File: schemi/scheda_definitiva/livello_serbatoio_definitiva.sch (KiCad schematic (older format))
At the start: 46 parts, among them J1 USB_B, J2 BTN_LED_GROUP, J3 CONN_LCD, J4 CONN_US, J5 ICSP, J6 Exp_Analog_2, J7 Exp_Analog, SW1 SW_RST, U1 FT232RL, U2 ATmega328P-PU, U3 USBLC6-2SC6, Y1 16MHz

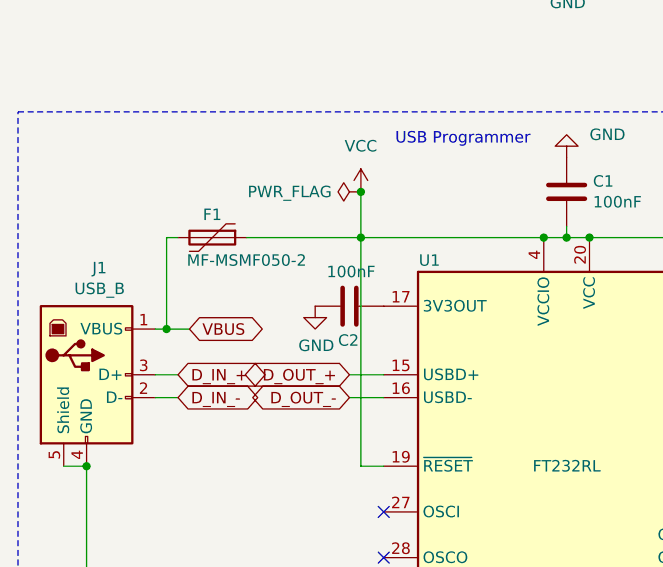
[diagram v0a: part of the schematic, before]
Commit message: aggiunta ferrite a scheda rev. B
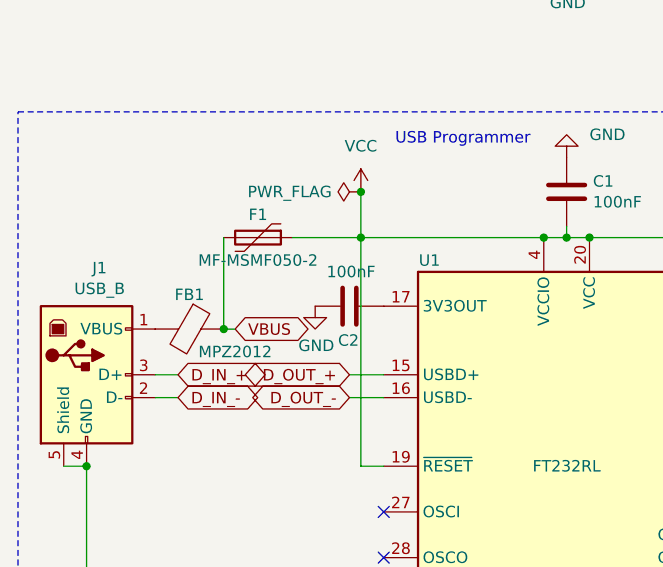
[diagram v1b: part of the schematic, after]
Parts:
- added FB1: MPZ2012, Inductor_SMD:L_0805_2012Metric_Pad1.15x1.40mm_HandSolder, symbol Device:Ferrite_Bead
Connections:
- net VBUS: now also FB1.1; no longer J1.1 (VBUS)
- new net: FB1.2, J1.1 (VBUS)
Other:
- moved on the sheet: F1
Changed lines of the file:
@@
 	0    -1   -1   0
 $EndComp
-Wire Wire Line
-	1250 2750 1300 2750
-Connection ~ 1300 2750
-Wire Wire Line
-	1300 2350 1300 2750
 $Comp
 L Device:R R9
@@
 DTR
 Wire Wire Line
-	1650 2350 2150 2350
-Wire Wire Line
 	2150 2150 2150 2350
 NoConn ~ 2250 3750
@@
 Wire Wire Line
 	2250 3350 2150 3350
-Wire Wire Line
-	1300 2350 1350 2350
 $Comp
 L Device:C C2
@@
 Text GLabel 1350 3050 2    50   BiDi ~ 0
 D_IN_-
-Text GLabel 1400 2750 2    50   BiDi ~ 0
-VBUS
 Text GLabel 2100 2950 0    50   BiDi ~ 0
 D_OUT_+
@@
 Text GLabel 2050 5700 2    50   BiDi ~ 0
 D_OUT_-
-Wire Wire Line
-	1300 2750 1400 2750
 Wire Wire Line
 	1250 2950 1350 2950
@@
 L Device:Polyfuse F1
 U 1 1 5FB200DA
-P 1500 2350
-F 0 "F1" V 1400 2350 50  0000 C CNN
-F 1 "MF-MSMF050-2" V 1600 2500 50  0000 C CNN
-F 2 "simboli_custom:MF-MSMF_1812_4532Metric_Pad1.30x3.40mm_HandSolder" H 1550 2150 50  0001 L CNN
-F 3 "~" H 1500 2350 50  0001 C CNN
-	1    1500 2350
+P 1700 2350
+F 0 "F1" V 1600 2350 50  0000 C CNN
+F 1 "MF-MSMF050-2" V 1800 2350 50  0000 C CNN
+F 2 "simboli_custom:MF-MSMF_1812_4532Metric_Pad1.30x3.40mm_HandSolder" H 1750 2150 50  0001 L CNN
+F 3 "~" H 1700 2350 50  0001 C CNN
+	1    1700 2350
 	0    1    1    0
 $EndComp
@@
 Wire Wire Line
 	4050 2350 4650 2350
+$Comp
+L Device:Ferrite_Bead FB1
+U 1 1 6044950F
+P 1400 2750
+F 0 "FB1" V 1250 2750 50  0000 C CNN
+F 1 "MPZ2012" V 1500 2950 50  0000 C CNN
+F 2 "Inductor_SMD:L_0805_2012Metric_Pad1.15x1.40mm_HandSolder" V 1330 2750 50  0001 C CNN
+F 3 "~" H 1400 2750 50  0001 C CNN
+	1    1400 2750
+	0    1    1    0
+$EndComp
+Text GLabel 1600 2750 2    50   BiDi ~ 0
+VBUS
+Wire Wire Line
+	1600 2750 1550 2750
+Connection ~ 1550 2750
+Wire Wire Line
+	1550 2350 1550 2750
+Wire Wire Line
+	1850 2350 2150 2350
 $EndSCHEMATC
